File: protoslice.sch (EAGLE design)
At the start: 31 parts

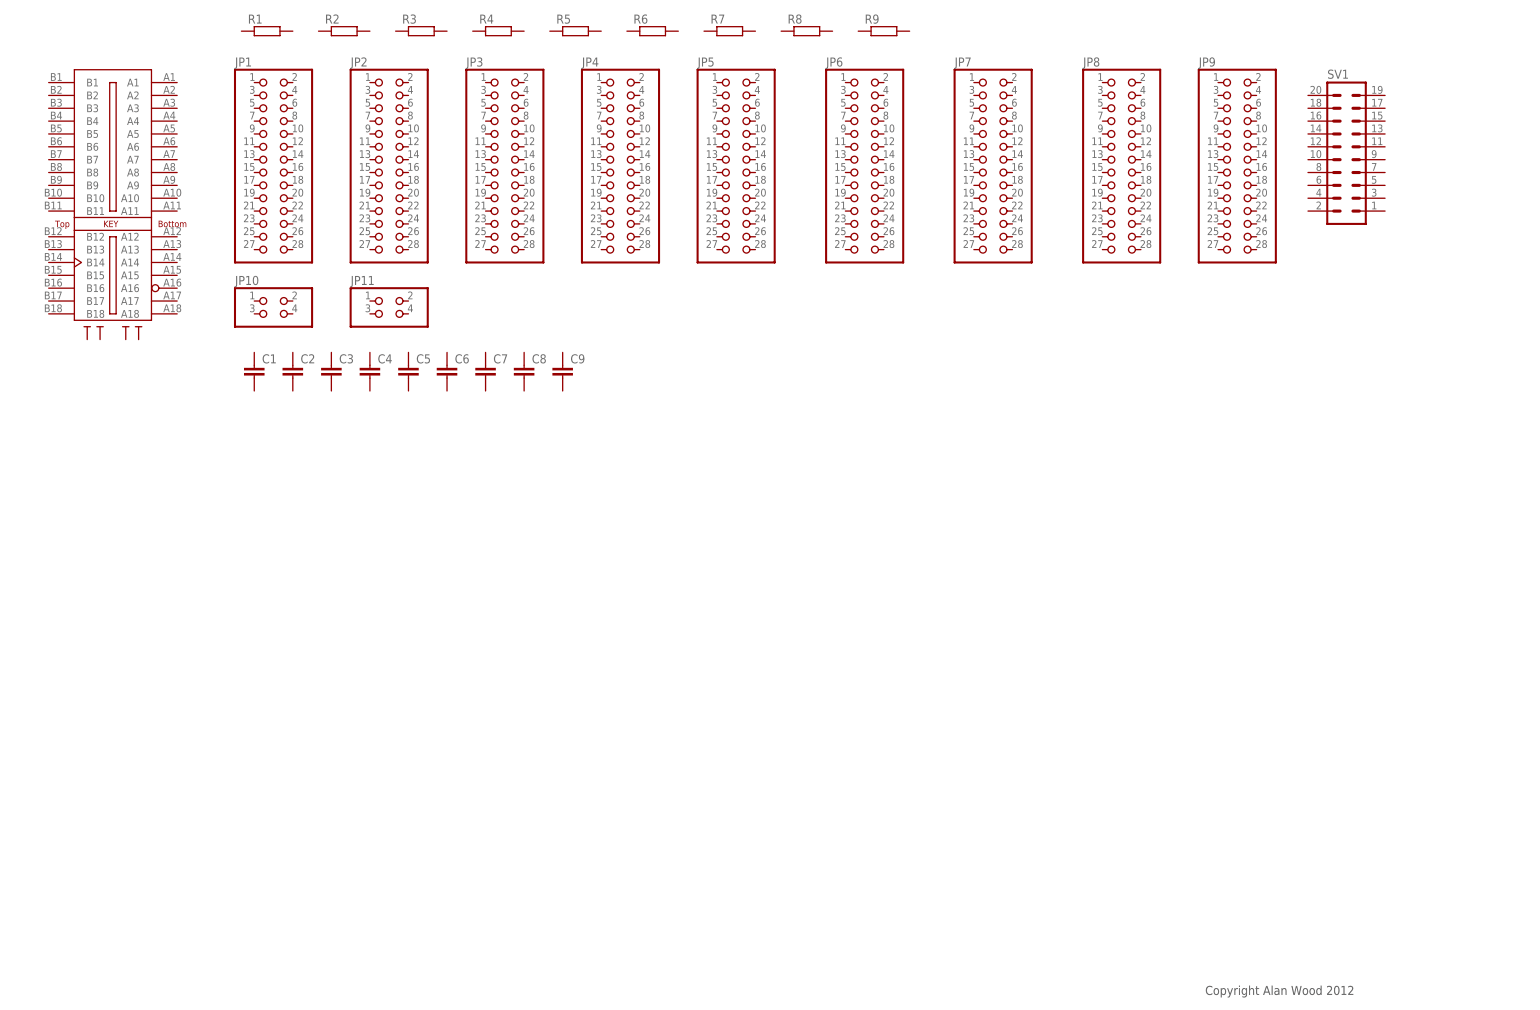
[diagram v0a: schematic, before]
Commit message: Made for energy monitor proto
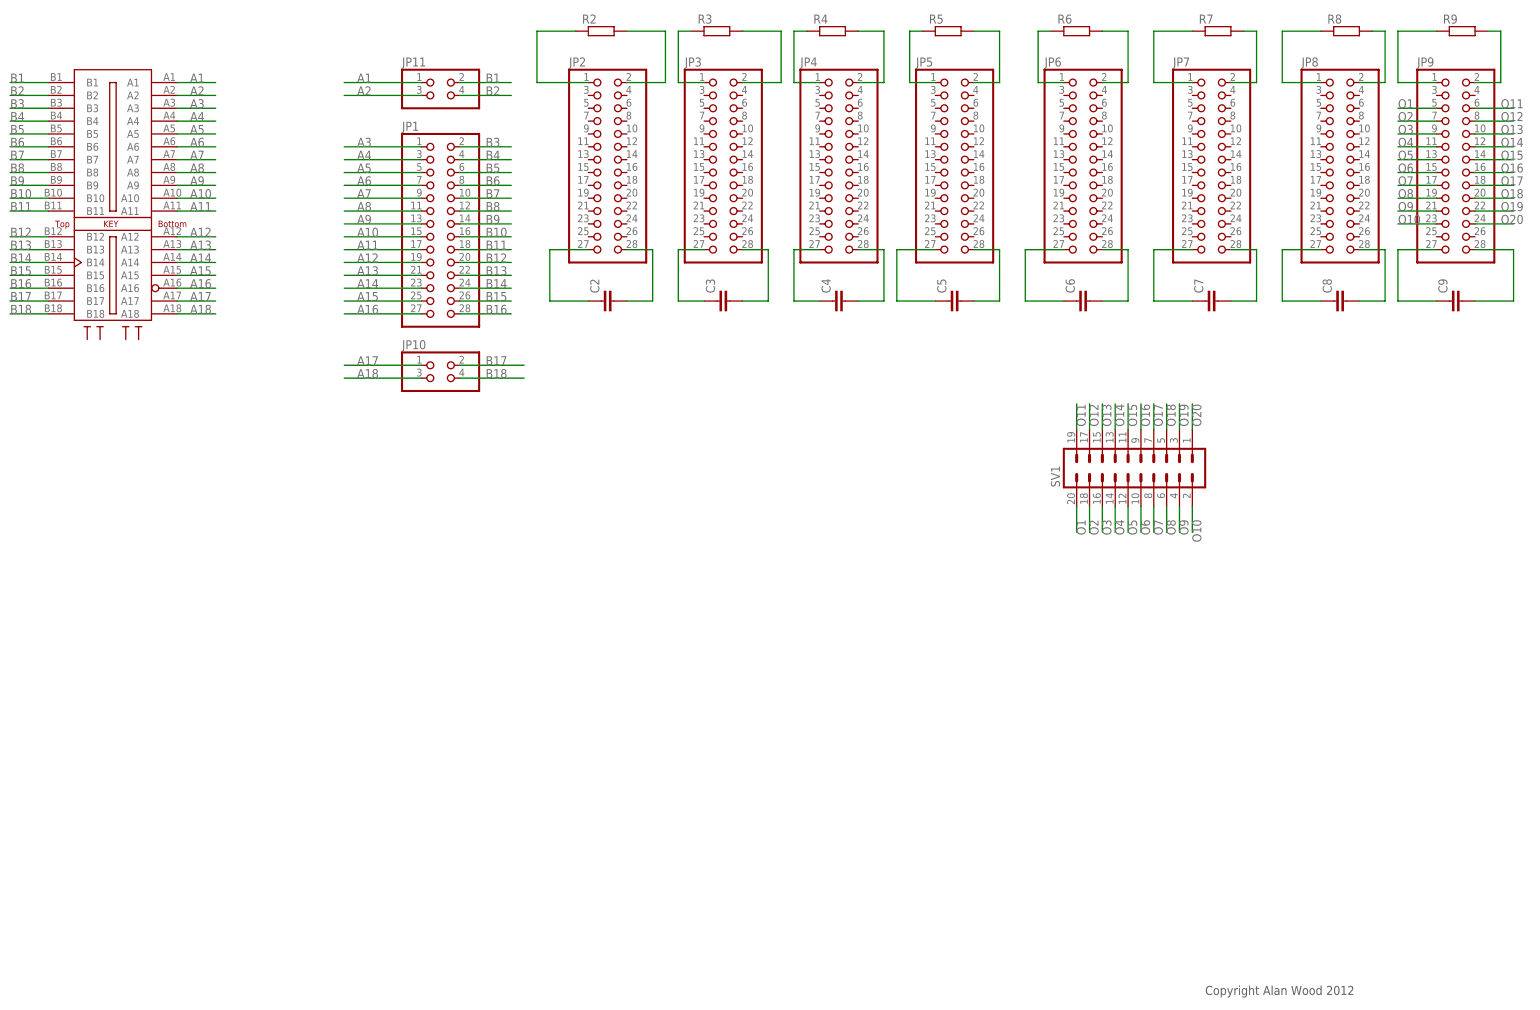
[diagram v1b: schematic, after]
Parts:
- removed C1: (no value), rcl:C-EUC0805
- removed R1: (no value), rcl:R-EU_R0805
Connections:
- new net A1: JP11.1, U$1.A1
- new net A10: JP1.15, U$1.A10
- new net A11: JP1.17, U$1.A11
- new net A12: JP1.19, U$1.A12
- new net A13: JP1.21, U$1.A13
- new net A14: JP1.23, U$1.A14
- new net A15: JP1.25, U$1.A15
- new net A16: JP1.27, U$1.A16
- new net A17: JP10.1, U$1.A17
- new net A18: JP10.3, U$1.A18
- new net A2: JP11.3, U$1.A2
- new net A3: JP1.1, U$1.A3
- new net A4: JP1.3, U$1.A4
- new net A5: JP1.5, U$1.A5
- new net A6: JP1.7, U$1.A6
- new net A7: JP1.9, U$1.A7
- new net A8: JP1.11, U$1.A8
- new net A9: JP1.13, U$1.A9
- new net B1: JP11.2, U$1.B1
- new net B10: JP1.16, U$1.B10
- new net B11: JP1.18, U$1.B11
- new net B12: JP1.20, U$1.B12
- new net B13: JP1.22, U$1.B13
- new net B14: JP1.24, U$1.B14
- new net B15: JP1.26, U$1.B15
- new net B16: JP1.28, U$1.B16
- new net B17: JP10.2, U$1.B17
- new net B18: JP10.4, U$1.B18
- new net B2: JP11.4, U$1.B2
- new net B3: JP1.2, U$1.B3
- new net B4: JP1.4, U$1.B4
- new net B5: JP1.6, U$1.B5
- new net B6: JP1.8, U$1.B6
- new net B7: JP1.10, U$1.B7
- new net B8: JP1.12, U$1.B8
- new net B9: JP1.14, U$1.B9
- new net N$1: JP2.1, R2.1
- new net N$10: JP5.2, R5.2
- new net N$11: JP6.1, R6.1
- new net N$12: JP6.2, R6.2
- new net N$13: JP7.1, R7.1
- new net N$14: JP7.2, R7.2
- new net N$15: C7.1, JP7.27
- new net N$16: C7.2, JP7.28
- new net N$17: C6.2, JP6.28
- new net N$18: C6.1, JP6.27
- new net N$19: C5.2, JP5.28
- new net N$2: JP2.2, R2.2
- new net N$20: C5.1, JP5.27
- new net N$21: C4.2, JP4.28
- new net N$22: C4.1, JP4.27
- new net N$23: C3.2, JP3.28
- new net N$24: C3.1, JP3.27
- new net N$25: JP8.1, R8.1
- new net N$26: JP8.2, R8.2
- new net N$27: C8.1, JP8.27
- new net N$28: C8.2, JP8.28
- new net N$29: C9.1, JP9.27
- new net N$3: C2.1, JP2.27
- new net N$30: C9.2, JP9.28
- new net N$31: JP9.1, R9.1
- new net N$32: JP9.2, R9.2
- new net N$4: C2.2, JP2.28
- new net N$5: JP3.1, R3.1
- new net N$6: JP3.2, R3.2
- new net N$7: JP4.1, R4.1
- new net N$8: JP4.2, R4.2
- new net N$9: JP5.1, R5.1
- new net O1: JP9.5, SV1.20
- new net O10: JP9.23, SV1.2
- new net O11: JP9.6, SV1.19
- new net O12: JP9.8, SV1.17
- new net O13: JP9.10, SV1.15
- new net O14: JP9.12, SV1.13
- new net O15: JP9.14, SV1.11
- new net O16: JP9.16, SV1.9
- new net O17: JP9.18, SV1.7
- new net O18: JP9.20, SV1.5
- new net O19: JP9.22, SV1.3
- new net O2: JP9.7, SV1.18
- new net O20: JP9.24, SV1.1
- new net O3: JP9.9, SV1.16
- new net O4: JP9.11, SV1.14
- new net O5: JP9.13, SV1.12
- new net O6: JP9.15, SV1.10
- new net O7: JP9.17, SV1.8
- new net O8: JP9.19, SV1.6
- new net O9: JP9.21, SV1.4
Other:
- moved on the sheet: C2, C3, C4, C5, C6, C7, C8, C9, JP1, JP10, JP11, JP2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
